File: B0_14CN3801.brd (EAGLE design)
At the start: 160 x 100 mm, 1 part

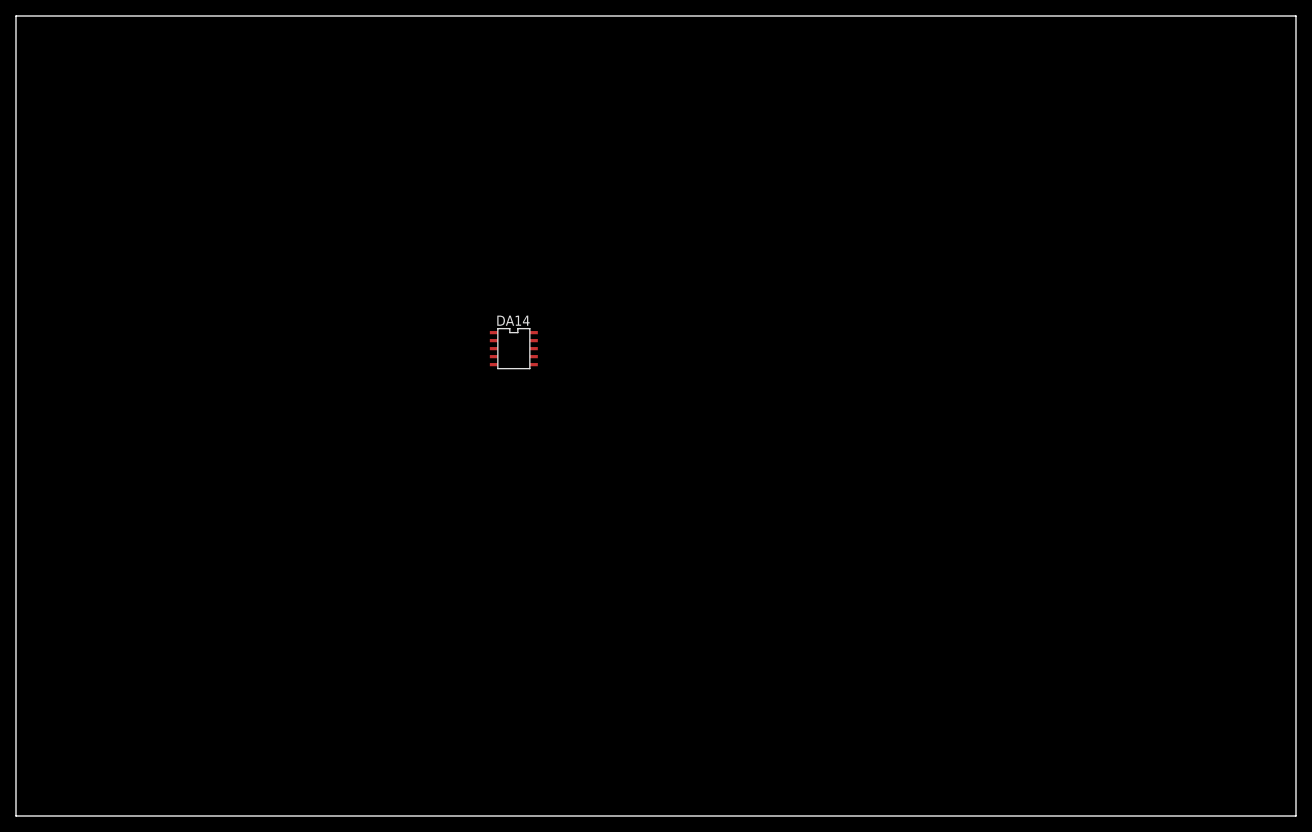
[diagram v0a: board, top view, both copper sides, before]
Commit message: .
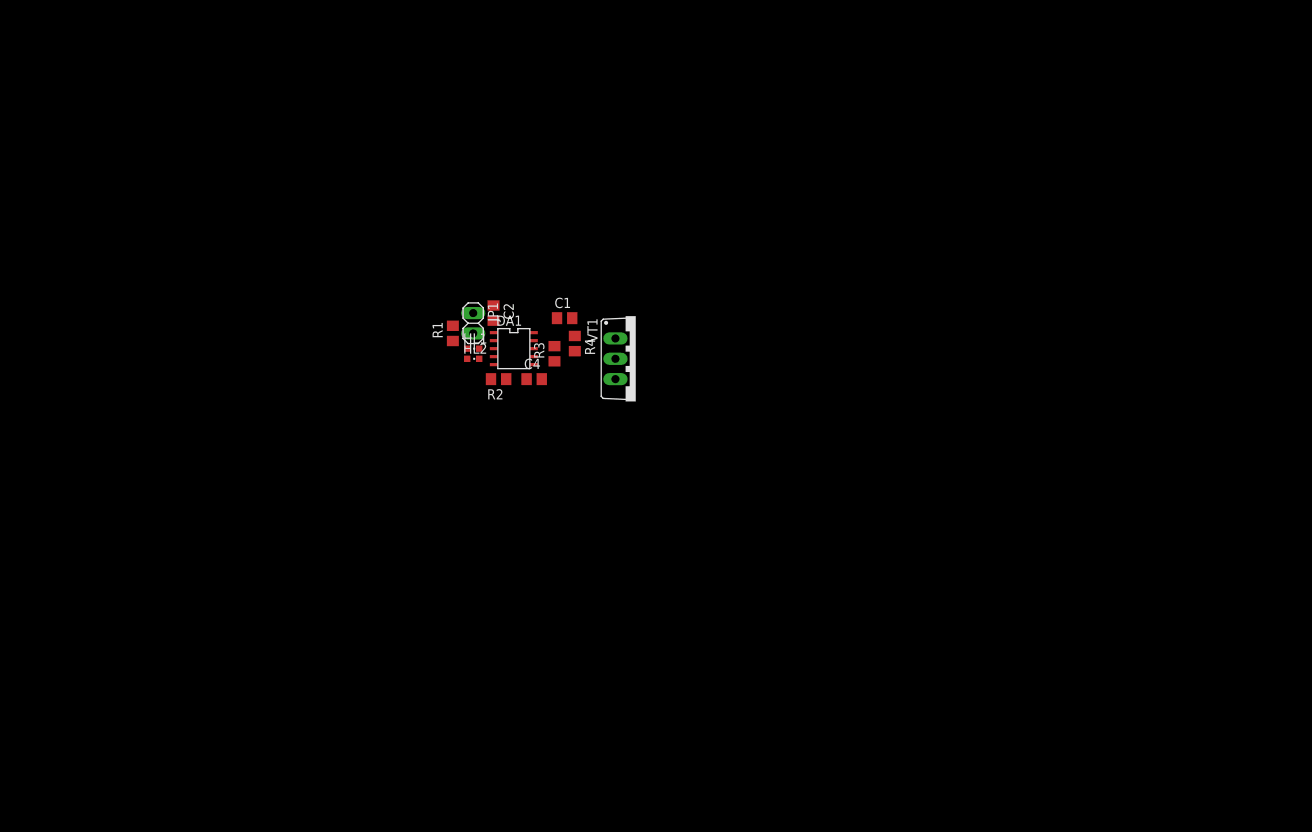
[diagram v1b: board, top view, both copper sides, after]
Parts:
- added C1, C2: 100n, rcl:C0805
- added C4: 220n, rcl:C0805
- added HL1, HL2: (no value), led:CHIPLED_0603
- added JP1: (no value), Разъёмы штырьковые 2.54мм:1X02
- added R1, R3, R4: (no value), rcl:R0805
- added R2: 120, rcl:R0805
- added VT1: (no value), m_transistor:TO220FV
- renumbered DA14 to DA1
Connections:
- removed net VCC: DA1.9
- new net N$1: C1.1, C2.1, DA1.9, JP1.1, R1.2, R3.2, VT1.3
- new net N$2: C2.2, DA1.1
- new net N$3: DA1.6, R3.1, R4.2
- new net N$4: DA1.5, R2.2
- new net N$5: HL1.A, HL2.A, R1.1
- new net N$6: DA1.3, HL1.C
- new net N$7: DA1.4, HL2.C
- new net N$8: C4.1, R2.1
- new net N$9: DA1.10, VT1.1
- net GND: now also C1.2, C4.2, JP1.2, R4.1
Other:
- board outline removed
